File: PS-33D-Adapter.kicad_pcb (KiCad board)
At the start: 2 copper layers, 15 x 7.6 mm, 8 parts, among them J1 CONN_05, J2 Conn_02x04_Counter_Clockwise, Q1 MOSFET-NCH-BSS138, Q2 MOSFET-NCH-BSS138

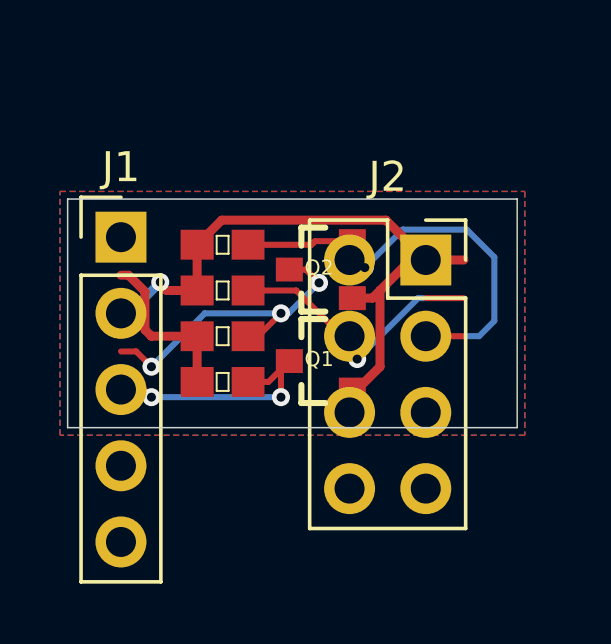
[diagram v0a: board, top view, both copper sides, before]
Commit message: feat: remove all traces
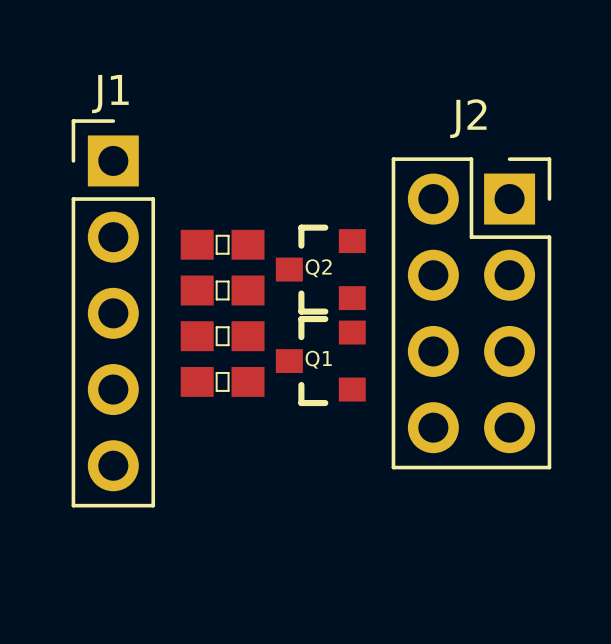
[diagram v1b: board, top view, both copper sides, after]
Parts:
- moved J2 3.45 mm to (160.3, 77.5)
- moved J1 2.55 mm to (147.1, 76.2)
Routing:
- net 3V3: track 21.2 -> 0.00 mm, vias 1 -> 0
- net SCL: track 13.2 -> 0.00 mm, vias 1 -> 0
- net SDA: track 10.7 -> 0.00 mm, vias 1 -> 0
- net M.SCL: track 10.6 -> 0.00 mm, vias 3 -> 0
- net M.SDA: track 8.42 -> 0.00 mm, vias 2 -> 0
- net 5V: track 5.65 -> 0.00 mm
- removed copper zone on B.Cu, net GND
- removed copper zone on F.Cu, net GND
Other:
- board outline removed
